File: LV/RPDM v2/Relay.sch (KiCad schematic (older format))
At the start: 4 parts

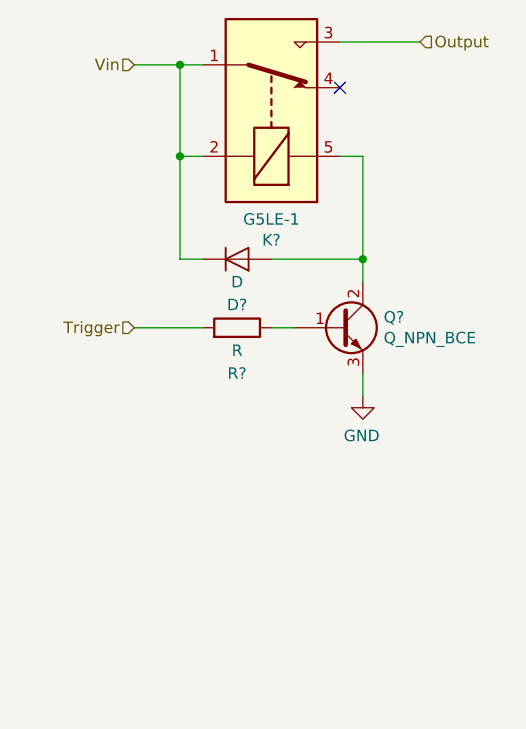
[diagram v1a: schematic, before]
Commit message: rpdm
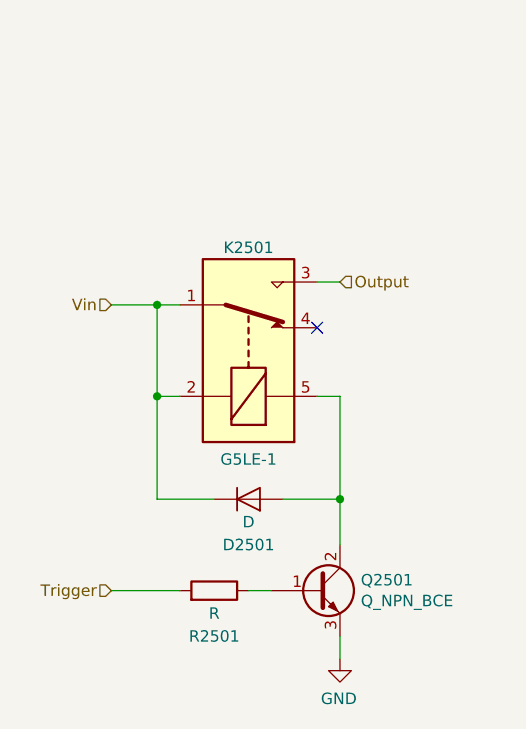
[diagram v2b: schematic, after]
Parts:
- gave numbers to parts that had none: 4
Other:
- moved on the sheet: D2501, K2501, Q2501, R2501
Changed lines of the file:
@@
 $Descr A4 11693 8268
 encoding utf-8
-Sheet 24 30
+Sheet 25 30
 Title "Relay Circuit"
 Date "2021-06-28"
@@
 L Relay:G5LE-1 K?
 U 1 1 5E5EE7C7
-P 5700 2100
+P 5600 3150
 AR Path="/5E554D5D/5E5EE7C7" Ref="K?"  Part="1"
-AR Path="/5E554D5D/5E5E9CA9/5E5EE7C7" Ref="K?"  Part="1"
+AR Path="/5E554D5D/5E5E9CA9/5E5EE7C7" Ref="K2501"  Part="1"
 AR Path="/5E554D5D/5E5A0290/5E5EE7C7" Ref="K?"  Part="1"
 AR Path="/5E554D5D/5E5A035E/5E5EE7C7" Ref="K?"  Part="1"
@@
 AR Path="/5E554D5D/60DE7B67/5E5EE7C7" Ref="K?"  Part="1"
 AR Path="/5E554D5D/60DE7FBD/5E5EE7C7" Ref="K?"  Part="1"
-AR Path="/5E554D5D/60DE88EB/5E5EE7C7" Ref="K?"  Part="1"
-AR Path="/5E554D5D/60DED789/5E5EE7C7" Ref="K?"  Part="1"
-AR Path="/5E554D5D/60DEDCB5/5E5EE7C7" Ref="K?"  Part="1"
-F 0 "K?" V 5133 2100 50  0000 C CNN
-F 1 "G5LE-1" V 5224 2100 50  0000 C CNN
-F 2 "Relay_THT:Relay_SPDT_Omron-G5LE-1" H 6150 2050 50  0001 L CNN
-F 3 "http://www.omron.com/ecb/products/pdf/en-g5le.pdf" H 5700 2100 50  0001 C CNN
-	1    5700 2100
+AR Path="/5E554D5D/60DE88EB/5E5EE7C7" Ref="K2201"  Part="1"
+AR Path="/5E554D5D/60DED789/5E5EE7C7" Ref="K2301"  Part="1"
+AR Path="/5E554D5D/60DEDCB5/5E5EE7C7" Ref="K2401"  Part="1"
+AR Path="/60E5EBEF/5E5EE7C7" Ref="K?"  Part="1"
+F 0 "K2501" V 6050 3150 50  0000 C CNN
+F 1 "G5LE-1" V 5124 3150 50  0000 C CNN
+F 2 "Relay_THT:Relay_SPDT_Omron-G5LE-1" H 6050 3100 50  0001 L CNN
+F 3 "http://www.omron.com/ecb/products/pdf/en-g5le.pdf" H 5600 3150 50  0001 C CNN
+	1    5600 3150
 	0    1    -1   0
 $EndComp
@@
 L Device:D D?
 U 1 1 5E5EE7CD
-P 5550 2750
+P 5600 3800
 AR Path="/5E554D5D/5E5EE7CD" Ref="D?"  Part="1"
-AR Path="/5E554D5D/5E5E9CA9/5E5EE7CD" Ref="D?"  Part="1"
+AR Path="/5E554D5D/5E5E9CA9/5E5EE7CD" Ref="D2501"  Part="1"
 AR Path="/5E554D5D/5E5A0290/5E5EE7CD" Ref="D?"  Part="1"
 AR Path="/5E554D5D/5E5A035E/5E5EE7CD" Ref="D?"  Part="1"
@@
 AR Path="/5E554D5D/60DE7B67/5E5EE7CD" Ref="D?"  Part="1"
 AR Path="/5E554D5D/60DE7FBD/5E5EE7CD" Ref="D?"  Part="1"
-AR Path="/5E554D5D/60DE88EB/5E5EE7CD" Ref="D?"  Part="1"
-AR Path="/5E554D5D/60DED789/5E5EE7CD" Ref="D?"  Part="1"
-AR Path="/5E554D5D/60DEDCB5/5E5EE7CD" Ref="D?"  Part="1"
-F 0 "D?" H 5550 2950 50  0000 C CNN
-F 1 "D" H 5550 2850 50  0000 C CNN
-F 2 "" H 5550 2750 50  0001 C CNN
-F 3 "~" H 5550 2750 50  0001 C CNN
-	1    5550 2750
+AR Path="/5E554D5D/60DE88EB/5E5EE7CD" Ref="D2201"  Part="1"
+AR Path="/5E554D5D/60DED789/5E5EE7CD" Ref="D2301"  Part="1"
+AR Path="/5E554D5D/60DEDCB5/5E5EE7CD" Ref="D2401"  Part="1"
+AR Path="/60E5EBEF/5E5EE7CD" Ref="D?"  Part="1"
+F 0 "D2501" H 5600 4000 50  0000 C CNN
+F 1 "D" H 5600 3900 50  0000 C CNN
+F 2 "" H 5600 3800 50  0001 C CNN
+F 3 "~" H 5600 3800 50  0001 C CNN
+	1    5600 3800
 	1    0    0    1
 $EndComp
 Wire Wire Line
-	5700 2750 6100 2750
+	5750 3800 6000 3800
 Wire Wire Line
-	6100 2750 6100 2300
+	6000 3800 6000 3350
 Wire Wire Line
-	6100 2300 6000 2300
+	6000 3350 5900 3350
 Wire Wire Line
-	5400 2300 5300 2300
+	5300 3350 5200 3350
 Wire Wire Line
-	5300 2300 5300 2750
+	5200 3350 5200 3800
 Wire Wire Line
-	5300 2750 5400 2750
-Text HLabel 5100 1900 0    50   Input ~ 0
+	5200 3800 5450 3800
+Text HLabel 5000 2950 0    50   Input ~ 0
 Vin
-NoConn ~ 6000 2000
-Text HLabel 6350 1800 2    50   Input ~ 0
+NoConn ~ 5900 3050
+Text HLabel 6000 2850 2    50   Input ~ 0
 Output
 $Comp
-L Device:Q_NPN_BCE Q?
+L Device:Q_NPN_BCE Q2501
 U 1 1 5E5F1342
-P 6000 3050
-AR Path="/5E554D5D/5E5E9CA9/5E5F1342" Ref="Q?"  Part="1"
+P 5900 4200
+AR Path="/5E554D5D/5E5E9CA9/5E5F1342" Ref="Q2501"  Part="1"
 AR Path="/5E554D5D/5E5A0290/5E5F1342" Ref="Q?"  Part="1"
 AR Path="/5E554D5D/5E5A035E/5E5F1342" Ref="Q?"  Part="1"
@@
 AR Path="/5E554D5D/60DE7B67/5E5F1342" Ref="Q?"  Part="1"
 AR Path="/5E554D5D/60DE7FBD/5E5F1342" Ref="Q?"  Part="1"
-AR Path="/5E554D5D/60DE88EB/5E5F1342" Ref="Q?"  Part="1"
-AR Path="/5E554D5D/60DED789/5E5F1342" Ref="Q?"  Part="1"
-AR Path="/5E554D5D/60DEDCB5/5E5F1342" Ref="Q?"  Part="1"
-F 0 "Q?" H 6191 3096 50  0000 L CNN
-F 1 "Q_NPN_BCE" H 6191 3005 50  0000 L CNN
-F 2 "" H 6200 3150 50  0001 C CNN
-F 3 "~" H 6000 3050 50  0001 C CNN
-	1    6000 3050
+AR Path="/5E554D5D/60DE88EB/5E5F1342" Ref="Q2201"  Part="1"
+AR Path="/5E554D5D/60DED789/5E5F1342" Ref="Q2301"  Part="1"
+AR Path="/5E554D5D/60DEDCB5/5E5F1342" Ref="Q2401"  Part="1"
+AR Path="/60E5EBEF/5E5F1342" Ref="Q?"  Part="1"
+F 0 "Q2501" H 6091 4246 50  0000 L CNN
+F 1 "Q_NPN_BCE" H 6091 4155 50  0000 L CNN
+F 2 "" H 6100 4300 50  0001 C CNN
+F 3 "~" H 5900 4200 50  0001 C CNN
+	1    5900 4200
 	1    0    0    -1
 $EndComp
 $Comp
-L Device:R R?
+L Device:R R2501
 U 1 1 5E5F2921
-P 5550 3050
-AR Path="/5E554D5D/5E5E9CA9/5E5F2921" Ref="R?"  Part="1"
+P 5450 4200
+AR Path="/5E554D5D/5E5E9CA9/5E5F2921" Ref="R2501"  Part="1"
 AR Path="/5E554D5D/5E5A0290/5E5F2921" Ref="R?"  Part="1"
 AR Path="/5E554D5D/5E5A035E/5E5F2921" Ref="R?"  Part="1"
@@
 AR Path="/5E554D5D/60DE7B67/5E5F2921" Ref="R?"  Part="1"
 AR Path="/5E554D5D/60DE7FBD/5E5F2921" Ref="R?"  Part="1"
-AR Path="/5E554D5D/60DE88EB/5E5F2921" Ref="R?"  Part="1"
-AR Path="/5E554D5D/60DED789/5E5F2921" Ref="R?"  Part="1"
-AR Path="/5E554D5D/60DEDCB5/5E5F2921" Ref="R?"  Part="1"
-F 0 "R?" V 5350 3050 50  0000 C CNN
-F 1 "R" V 5450 3050 50  0000 C CNN
-F 2 "" V 5480 3050 50  0001 C CNN
-F 3 "~" H 5550 3050 50  0001 C CNN
-	1    5550 3050
+AR Path="/5E554D5D/60DE88EB/5E5F2921" Ref="R2201"  Part="1"
+AR Path="/5E554D5D/60DED789/5E5F2921" Ref="R2301"  Part="1"
+AR Path="/5E554D5D/60DEDCB5/5E5F2921" Ref="R2401"  Part="1"
+AR Path="/60E5EBEF/5E5F2921" Ref="R?"  Part="1"
+F 0 "R2501" V 5250 4200 50  0000 C CNN
+F 1 "R" V 5350 4200 50  0000 C CNN
+F 2 "" V 5380 4200 50  0001 C CNN
+F 3 "~" H 5450 4200 50  0001 C CNN
+	1    5450 4200
 	0    1    -1   0
 $EndComp
 Wire Wire Line
-	6000 1800 6350 1800
+	5900 2850 6000 2850
 $Comp
-L power:GND #PWR?
+L power:GND #PWR02501
 U 1 1 5E5F4802
-P 6100 3350
-AR Path="/5E554D5D/5E5E9CA9/5E5F4802" Ref="#PWR?"  Part="1"
+P 6000 4500
+AR Path="/5E554D5D/5E5E9CA9/5E5F4802" Ref="#PWR02501"  Part="1"
 AR Path="/5E554D5D/5E5A0290/5E5F4802" Ref="#PWR?"  Part="1"
 AR Path="/5E554D5D/5E5A035E/5E5F4802" Ref="#PWR?"  Part="1"
@@
 AR Path="/5E554D5D/60DE7B67/5E5F4802" Ref="#PWR?"  Part="1"
 AR Path="/5E554D5D/60DE7FBD/5E5F4802" Ref="#PWR?"  Part="1"
-AR Path="/5E554D5D/60DE88EB/5E5F4802" Ref="#PWR?"  Part="1"
-AR Path="/5E554D5D/60DED789/5E5F4802" Ref="#PWR?"  Part="1"
-AR Path="/5E554D5D/60DEDCB5/5E5F4802" Ref="#PWR?"  Part="1"
-F 0 "#PWR?" H 6100 3100 50  0001 C CNN
-F 1 "GND" H 6105 3177 50  0000 C CNN
-F 2 "" H 6100 3350 50  0001 C CNN
-F 3 "" H 6100 3350 50  0001 C CNN
-	1    6100 3350
+AR Path="/5E554D5D/60DE88EB/5E5F4802" Ref="#PWR02201"  Part="1"
+AR Path="/5E554D5D/60DED789/5E5F4802" Ref="#PWR02301"  Part="1"
+AR Path="/5E554D5D/60DEDCB5/5E5F4802" Ref="#PWR02401"  Part="1"
+AR Path="/60E5EBEF/5E5F4802" Ref="#PWR?"  Part="1"
+F 0 "#PWR02501" H 6000 4250 50  0001 C CNN
+F 1 "GND" H 6005 4327 50  0000 C CNN
+F 2 "" H 6000 4500 50  0001 C CNN
+F 3 "" H 6000 4500 50  0001 C CNN
+	1    6000 4500
 	-1   0    0    -1
 $EndComp
-Connection ~ 5300 2300
+Connection ~ 5200 3350
 Wire Wire Line
-	5100 1900 5300 1900
+	5000 2950 5200 2950
 Wire Wire Line
-	5300 1900 5300 2300
-Text HLabel 5100 3050 0    50   Input ~ 0
+	5200 2950 5200 3350
+Text HLabel 5000 4200 0    50   Input ~ 0
 Trigger
 Wire Wire Line
-	5400 1900 5300 1900
-Connection ~ 5300 1900
+	5300 2950 5200 2950
+Connection ~ 5200 2950
 Wire Wire Line
-	6100 3350 6100 3250
+	6000 4500 6000 4400
 Wire Wire Line
-	6100 2850 6100 2750
-Connection ~ 6100 2750
+	6000 4000 6000 3800
+Connection ~ 6000 3800
 Wire Wire Line
-	5800 3050 5700 3050
+	5700 4200 5600 4200
 Wire Wire Line
-	5400 3050 5100 3050
+	5300 4200 5000 4200
 $EndSCHEMATC
